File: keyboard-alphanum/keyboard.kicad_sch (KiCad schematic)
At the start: 173 parts, among them J1 USB_B_Mini, U1 ATmega168PA-A, U2 CH340C, U3 74HC154D, U4 74HC4051, Y1 16MHz

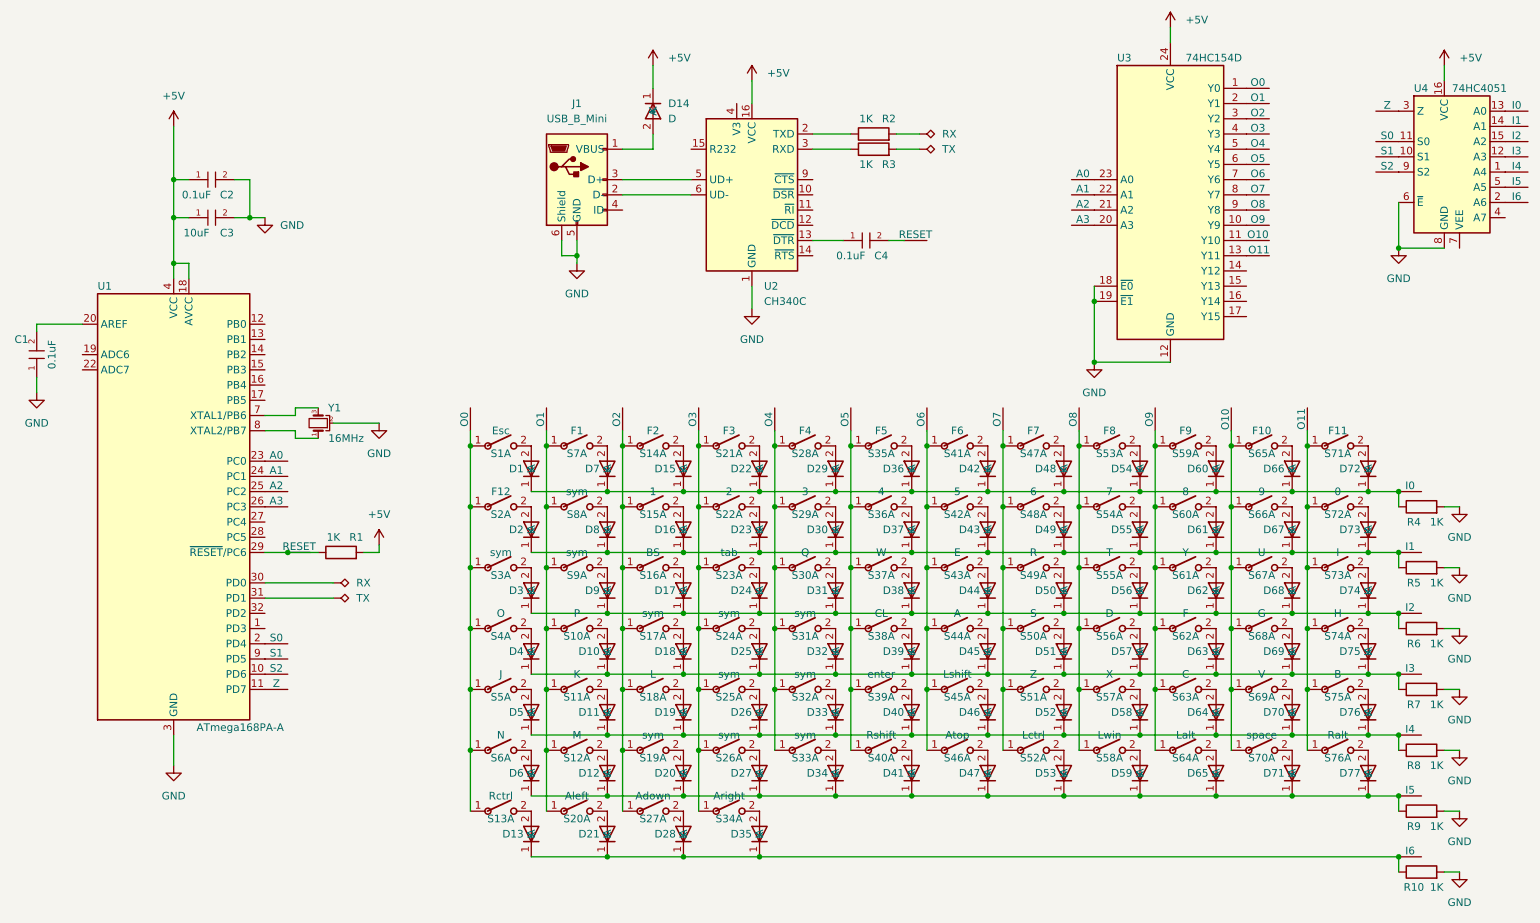
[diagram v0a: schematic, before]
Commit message: Keyboard alphanum v1.0
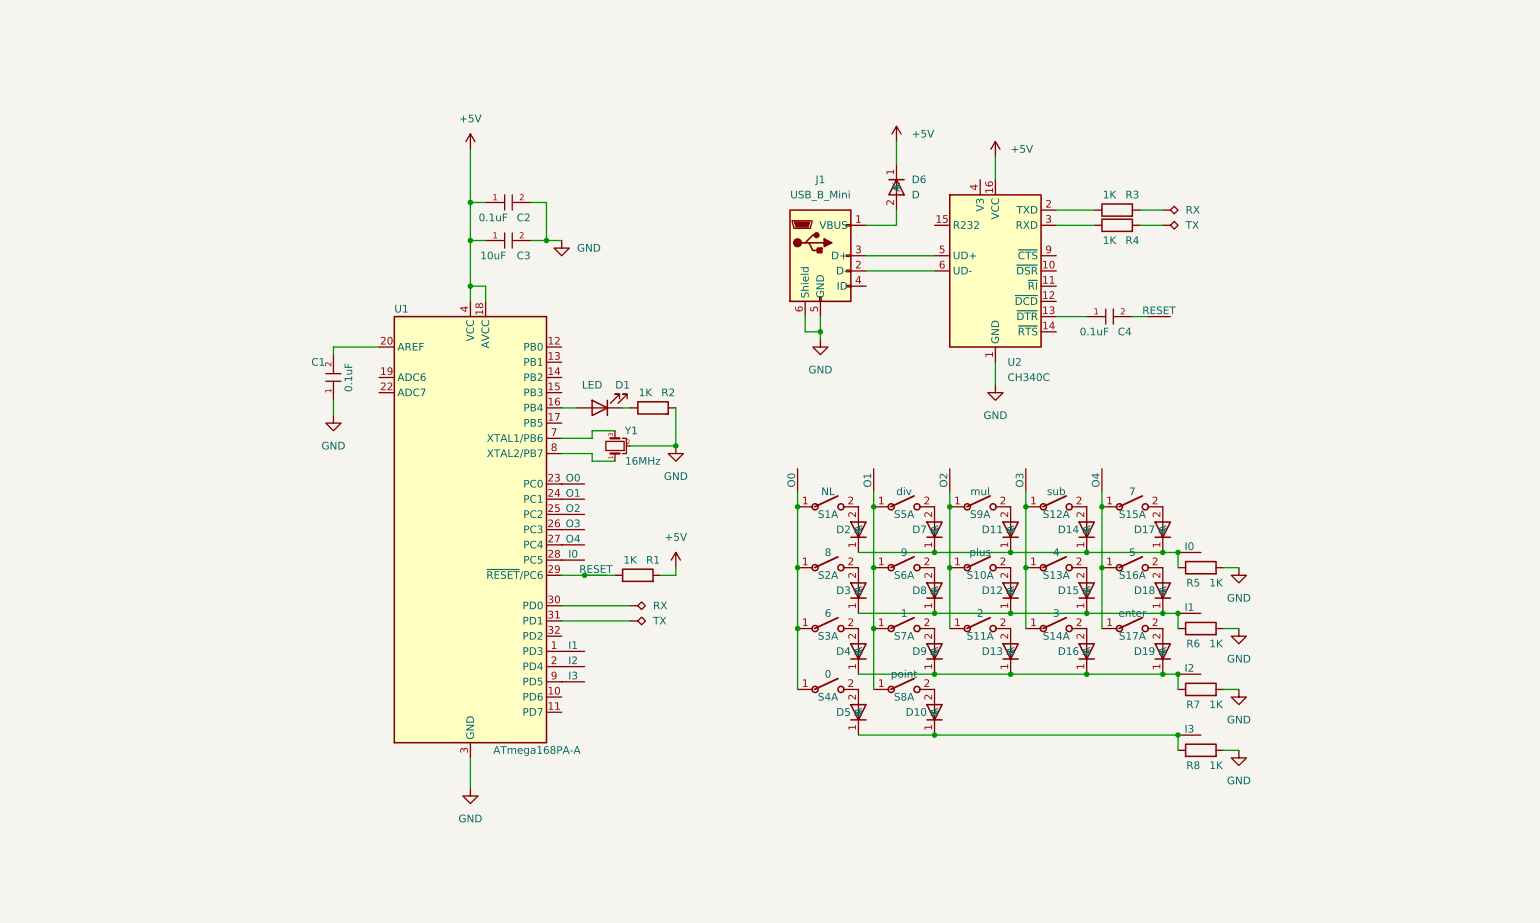
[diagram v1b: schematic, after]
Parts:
- removed D11, D12, D13, D18, D19, D20, D21, D25, D26, D27, D28, D32, D33, D34, D35, D36, D37, D38, D39, D40, D41, D42, D43, D44, D45, D46, D47, D48, D49, D5, D50, D51, D52, D53, D54, D55, D56, D57, D58, D59, D6, D60, D61, D62, D63, D64, D65, D66, D67, D68, D69, D70, D71, D72, D73, D74, D75, D76, D77: D, common:D_0603_1608Metric, symbol symbols:D
- removed R10, R8, R9: 1K, common:R_0603_1608Metric, symbol symbols:R
- removed S11: K, Switch_Keyboard_Cherry_MX:SW_Cherry_MX_PCB_1.00u, symbol symbols:Switch
- removed S12: M, Switch_Keyboard_Cherry_MX:SW_Cherry_MX_PCB_1.00u, symbol symbols:Switch
- removed S13: Rctrl, Switch_Keyboard_Cherry_MX:SW_Cherry_MX_PCB_1.00u, symbol symbols:Switch
- removed S17, S19, S24, S25, S26, S31, S32, S33: sym, Switch_Keyboard_Cherry_MX:SW_Cherry_MX_PCB_1.00u, symbol symbols:Switch
- removed S18: L, Switch_Keyboard_Cherry_MX:SW_Cherry_MX_PCB_1.00u, symbol symbols:Switch
- removed S20: Aleft, Switch_Keyboard_Cherry_MX:SW_Cherry_MX_PCB_1.00u, symbol symbols:Switch
- removed S27: Adown, Switch_Keyboard_Cherry_MX:SW_Cherry_MX_PCB_1.00u, symbol symbols:Switch
- removed S34: Aright, Switch_Keyboard_Cherry_MX:SW_Cherry_MX_PCB_1.00u, symbol symbols:Switch
- removed S35: F5, Switch_Keyboard_Cherry_MX:SW_Cherry_MX_PCB_1.00u, symbol symbols:Switch
- removed S36: 4, Switch_Keyboard_Cherry_MX:SW_Cherry_MX_PCB_1.00u, symbol symbols:Switch
- removed S37: W, Switch_Keyboard_Cherry_MX:SW_Cherry_MX_PCB_1.00u, symbol symbols:Switch
- removed S38: CL, Switch_Keyboard_Cherry_MX:SW_Cherry_MX_PCB_1.00u, symbol symbols:Switch
- removed S39: enter, Switch_Keyboard_Cherry_MX:SW_Cherry_MX_PCB_2.00u, symbol symbols:Switch
- removed S40: Rshift, Switch_Keyboard_Cherry_MX:SW_Cherry_MX_PCB_1.00u, symbol symbols:Switch
- removed S41: F6, Switch_Keyboard_Cherry_MX:SW_Cherry_MX_PCB_1.00u, symbol symbols:Switch
- removed S42: 5, Switch_Keyboard_Cherry_MX:SW_Cherry_MX_PCB_1.00u, symbol symbols:Switch
- removed S43: E, Switch_Keyboard_Cherry_MX:SW_Cherry_MX_PCB_1.00u, symbol symbols:Switch
- removed S44: A, Switch_Keyboard_Cherry_MX:SW_Cherry_MX_PCB_1.00u, symbol symbols:Switch
- removed S45: Lshift, Switch_Keyboard_Cherry_MX:SW_Cherry_MX_PCB_1.00u, symbol symbols:Switch
- removed S46: Atop, Switch_Keyboard_Cherry_MX:SW_Cherry_MX_PCB_1.00u, symbol symbols:Switch
- removed S47: F7, Switch_Keyboard_Cherry_MX:SW_Cherry_MX_PCB_1.00u, symbol symbols:Switch
- removed S48: 6, Switch_Keyboard_Cherry_MX:SW_Cherry_MX_PCB_1.00u, symbol symbols:Switch
- removed S49: R, Switch_Keyboard_Cherry_MX:SW_Cherry_MX_PCB_1.00u, symbol symbols:Switch
- removed S5: J, Switch_Keyboard_Cherry_MX:SW_Cherry_MX_PCB_1.00u, symbol symbols:Switch
- removed S50: S, Switch_Keyboard_Cherry_MX:SW_Cherry_MX_PCB_1.00u, symbol symbols:Switch
- removed S51: Z, Switch_Keyboard_Cherry_MX:SW_Cherry_MX_PCB_1.00u, symbol symbols:Switch
- removed S52: Lctrl, Switch_Keyboard_Cherry_MX:SW_Cherry_MX_PCB_1.00u, symbol symbols:Switch
- removed S53: F8, Switch_Keyboard_Cherry_MX:SW_Cherry_MX_PCB_1.00u, symbol symbols:Switch
- removed S54: 7, Switch_Keyboard_Cherry_MX:SW_Cherry_MX_PCB_1.00u, symbol symbols:Switch
- removed S55: T, Switch_Keyboard_Cherry_MX:SW_Cherry_MX_PCB_1.00u, symbol symbols:Switch
- removed S56: D, Switch_Keyboard_Cherry_MX:SW_Cherry_MX_PCB_1.00u, symbol symbols:Switch
- removed S57: X, Switch_Keyboard_Cherry_MX:SW_Cherry_MX_PCB_1.00u, symbol symbols:Switch
- removed S58: Lwin, Switch_Keyboard_Cherry_MX:SW_Cherry_MX_PCB_1.00u, symbol symbols:Switch
- removed S59: F9, Switch_Keyboard_Cherry_MX:SW_Cherry_MX_PCB_1.00u, symbol symbols:Switch
- removed S6: N, Switch_Keyboard_Cherry_MX:SW_Cherry_MX_PCB_1.00u, symbol symbols:Switch
- removed S60: 8, Switch_Keyboard_Cherry_MX:SW_Cherry_MX_PCB_1.00u, symbol symbols:Switch
- removed S61: Y, Switch_Keyboard_Cherry_MX:SW_Cherry_MX_PCB_1.00u, symbol symbols:Switch
- removed S62: F, Switch_Keyboard_Cherry_MX:SW_Cherry_MX_PCB_1.00u, symbol symbols:Switch
- removed S63: C, Switch_Keyboard_Cherry_MX:SW_Cherry_MX_PCB_1.00u, symbol symbols:Switch
- removed S64: Lalt, Switch_Keyboard_Cherry_MX:SW_Cherry_MX_PCB_1.00u, symbol symbols:Switch
- removed S65: F10, Switch_Keyboard_Cherry_MX:SW_Cherry_MX_PCB_1.00u, symbol symbols:Switch
- removed S66: 9, Switch_Keyboard_Cherry_MX:SW_Cherry_MX_PCB_1.00u, symbol symbols:Switch
- removed S67: U, Switch_Keyboard_Cherry_MX:SW_Cherry_MX_PCB_1.00u, symbol symbols:Switch
- removed S68: G, Switch_Keyboard_Cherry_MX:SW_Cherry_MX_PCB_1.00u, symbol symbols:Switch
- removed S69: V, Switch_Keyboard_Cherry_MX:SW_Cherry_MX_PCB_1.00u, symbol symbols:Switch
- removed S70: space, Switch_Keyboard_Cherry_MX:SW_Cherry_MX_PCB_6.00u, symbol symbols:Switch
- removed S71: F11, Switch_Keyboard_Cherry_MX:SW_Cherry_MX_PCB_1.00u, symbol symbols:Switch
- removed S72: 0, Switch_Keyboard_Cherry_MX:SW_Cherry_MX_PCB_1.00u, symbol symbols:Switch
- removed S73: I, Switch_Keyboard_Cherry_MX:SW_Cherry_MX_PCB_1.00u, symbol symbols:Switch
- removed S74: H, Switch_Keyboard_Cherry_MX:SW_Cherry_MX_PCB_1.00u, symbol symbols:Switch
- removed S75: B, Switch_Keyboard_Cherry_MX:SW_Cherry_MX_PCB_1.00u, symbol symbols:Switch
- removed S76: Ralt, Switch_Keyboard_Cherry_MX:SW_Cherry_MX_PCB_1.00u, symbol symbols:Switch
- removed U3: 74HC154D, common:SSOP-24_3.9x8.7mm_P0.635mm, symbol symbols:74HC154D
- removed U4: 74HC4051, common:SSOP-16_3.9x4.9mm_P0.635mm, symbol symbols:74HC4051
- added D1: LED, common:LED_1206_3216Metric, symbol symbols:LED
- added R2: 1K, common:R_0603_1608Metric, symbol symbols:R
- S1: value Esc -> NL
- S10: renamed from S15; value 1 -> plus; footprint Switch_Keyboard_Cherry_MX:SW_Cherry_MX_PCB_1.00u -> Switch_Keyboard_Cherry_MX:SW_Cherry_MX_PCB_2.00u_90deg
- S11: renamed from S16; value BS -> 2
- S12: renamed from S21; value F3 -> sub
- S13: renamed from S22; value 2 -> 4
- S14: renamed from S23; value tab -> 3
- S15: renamed from S28; value F4 -> 7
- S16: renamed from S29; value 3 -> 5
- S17: renamed from S30; value Q -> enter; footprint Switch_Keyboard_Cherry_MX:SW_Cherry_MX_PCB_1.00u -> Switch_Keyboard_Cherry_MX:SW_Cherry_MX_PCB_2.00u_90deg
- S2: value F12 -> 8
- S3: value sym -> 6
- S4: value O -> 0; footprint Switch_Keyboard_Cherry_MX:SW_Cherry_MX_PCB_1.00u -> Switch_Keyboard_Cherry_MX:SW_Cherry_MX_PCB_2.00u
- S5: renamed from S7; value F1 -> div
- S6: renamed from S8; value sym -> 9
- S7: renamed from S9; value sym -> 1
- S8: renamed from S10; value P -> point
- S9: renamed from S14; value F2 -> mul
- renumbered D15 to D11, D16 to D12, D17 to D13, D22 to D14, D23 to D15, D24 to D16, D29 to D17, D30 to D18, D31 to D19, D1 to D2, D2 to D3, D3 to D4, D4 to D5, D14 to D6, R2 to R3, R3 to R4, R4 to R5, R5 to R6, R6 to R7, R7 to R8
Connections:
- net GND: now also R2.2
- net I0: now also U1.28 (PC5)
- net I1: now also U1.1 (PD3)
- net I2: now also U1.2 (PD4)
- net I3: now also U1.9 (PD5)
- net O0: now also U1.23 (PC0)
- net O1: now also U1.24 (PC1)
- net O2: now also U1.25 (PC2)
- net O3: now also U1.26 (PC3)
- net O4: now also U1.27 (PC4)
- net at U1.16 (PB4): now also D1.2 (A)
- new net: D1.1 (K), R2.1
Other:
- title: Arduino Keyboard -> keyboard alphanum
- moved on the sheet: C1, C2, C3, C4, D10, D11, D12, D13, D14, D15, D16, D17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
